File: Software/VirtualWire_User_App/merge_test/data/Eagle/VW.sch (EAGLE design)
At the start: 5 parts

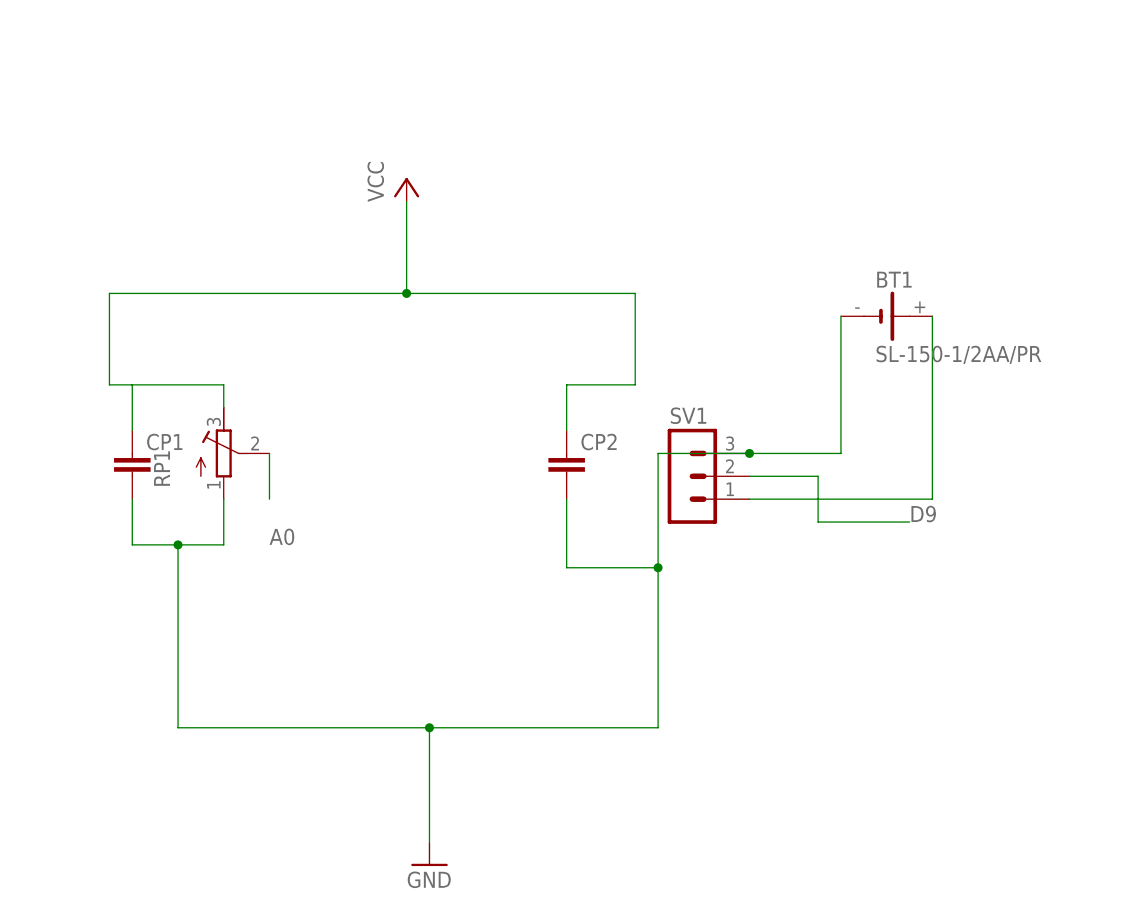
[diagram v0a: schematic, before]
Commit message: bug fixes
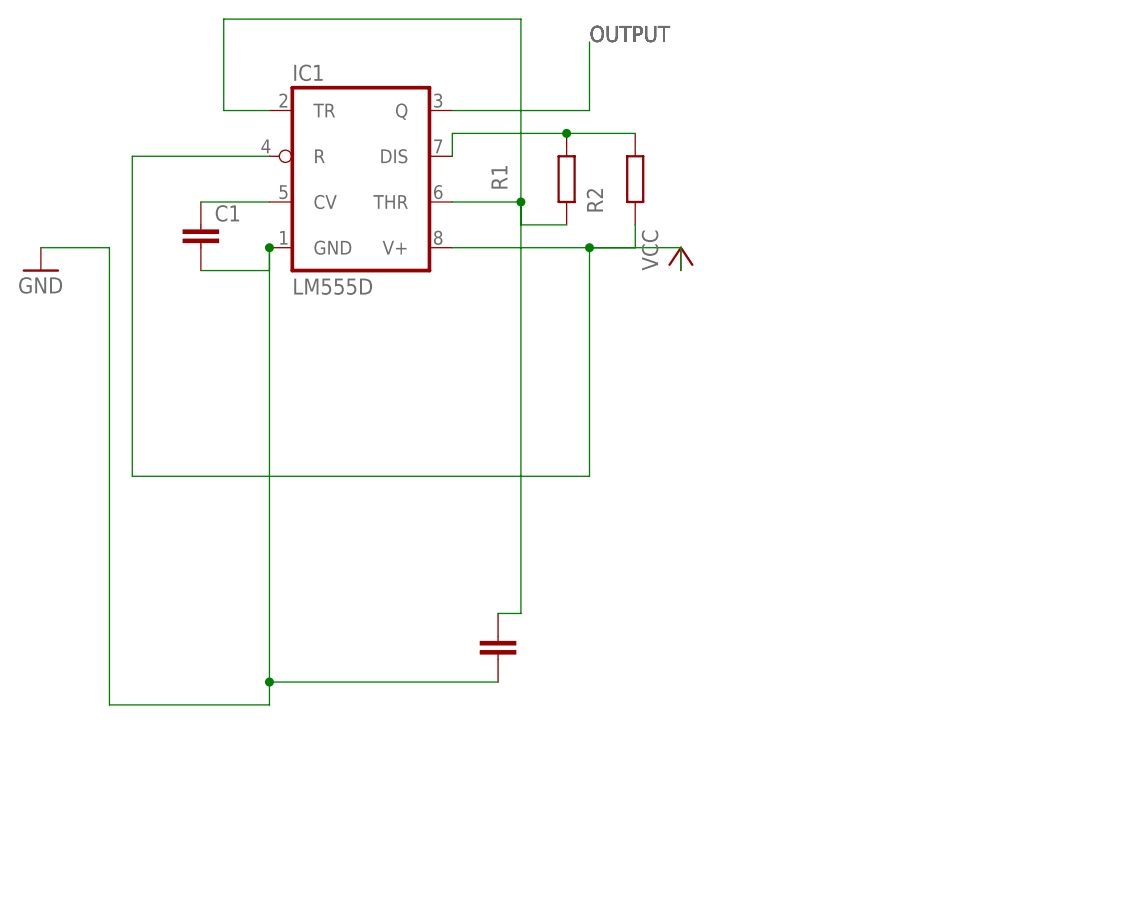
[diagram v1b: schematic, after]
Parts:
- removed BT1: SL-150-1/2AA/PR, battery:SL-150-1/2AA/PR
- removed CP1, CP2: (no value), capacitor-wima:C2,5-3
- removed RP1: (no value), rcl:R-TRIMM4G/J
- removed SV1: (no value), con-lstb:MA03-1
- added C1, C3: (no value), rcl:C-EU025-024X044
- added IC1: LM555D, linear:LM555D
- added R1, R2: (no value), rcl:R-EU_0204/5
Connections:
- removed net A0: RP1.S
- removed net A5V: CP1.1, CP2.1, RP1.E
- removed net D9: SV1.2
- removed net GND1: BT1.-, CP1.2, CP2.2, RP1.A, SV1.3
- new net GND: C1.2, C3.2, IC1.GND
- new net N$1: IC1.DIS, R1.2, R2.1
- new net N$6: C1.1, IC1.CV
- new net OUTPUT: IC1.Q
- new net VCC: IC1.R, IC1.V+, R2.2
- net N$2: now also C3.1, IC1.THR, IC1.TR, R1.1; no longer BT1.+, SV1.1
